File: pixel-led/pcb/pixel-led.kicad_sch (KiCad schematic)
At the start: 16 parts, among them J1 Conn_01x04_Socket, J2 USB_A, SW2 SW_Push, U1 AMS1117-3.3, U2 TSOP45xx, U3 ESP32-S3-MINI-1U, U4 USBLC6-2SC6

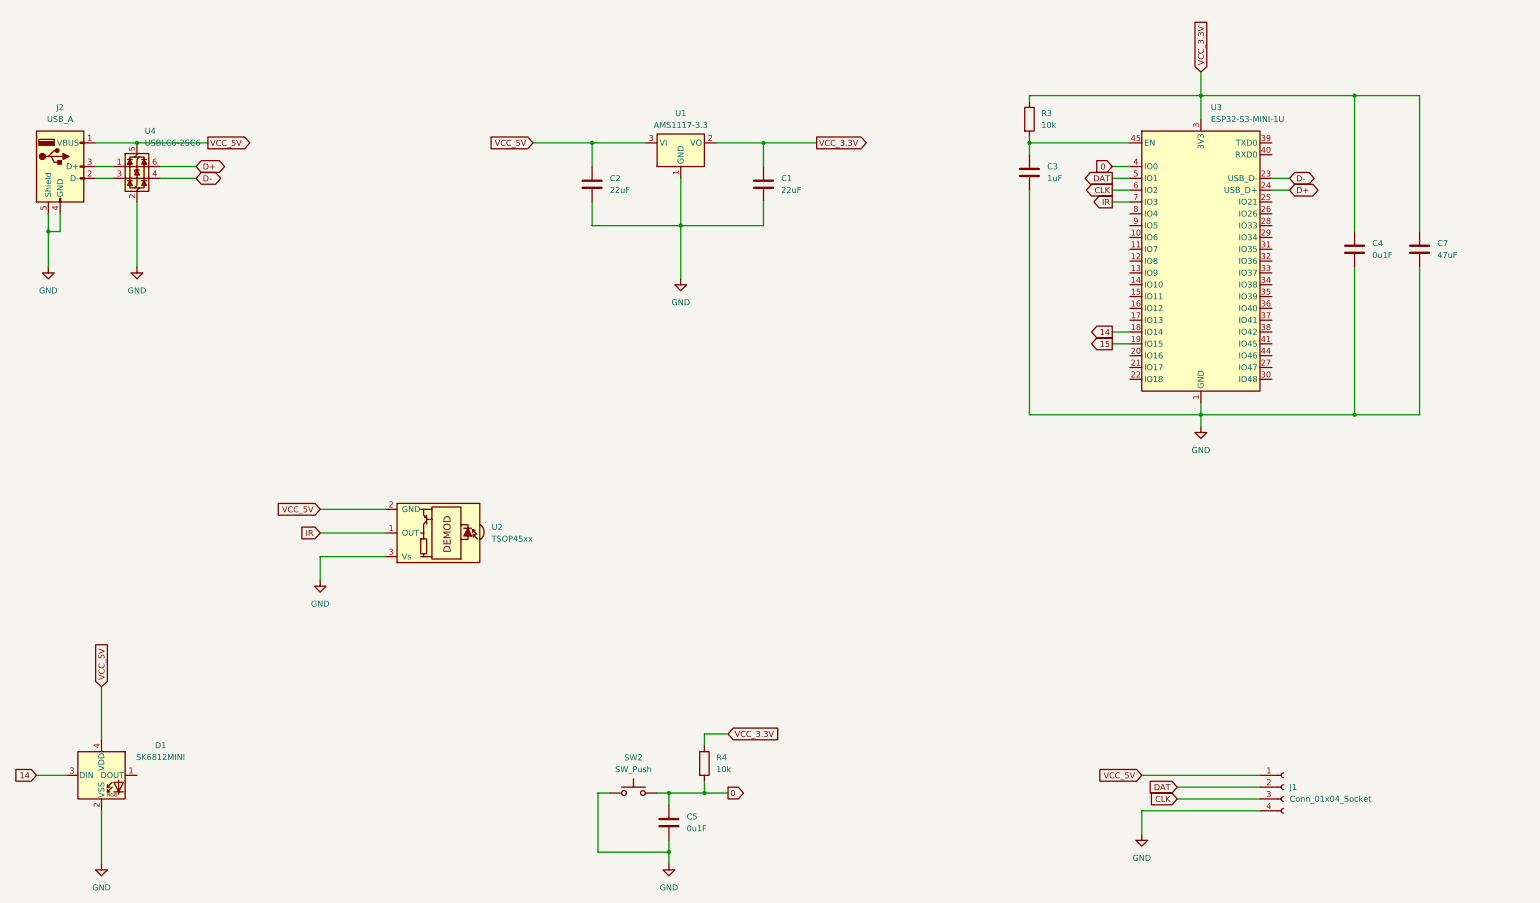
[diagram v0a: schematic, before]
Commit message: finishing layout
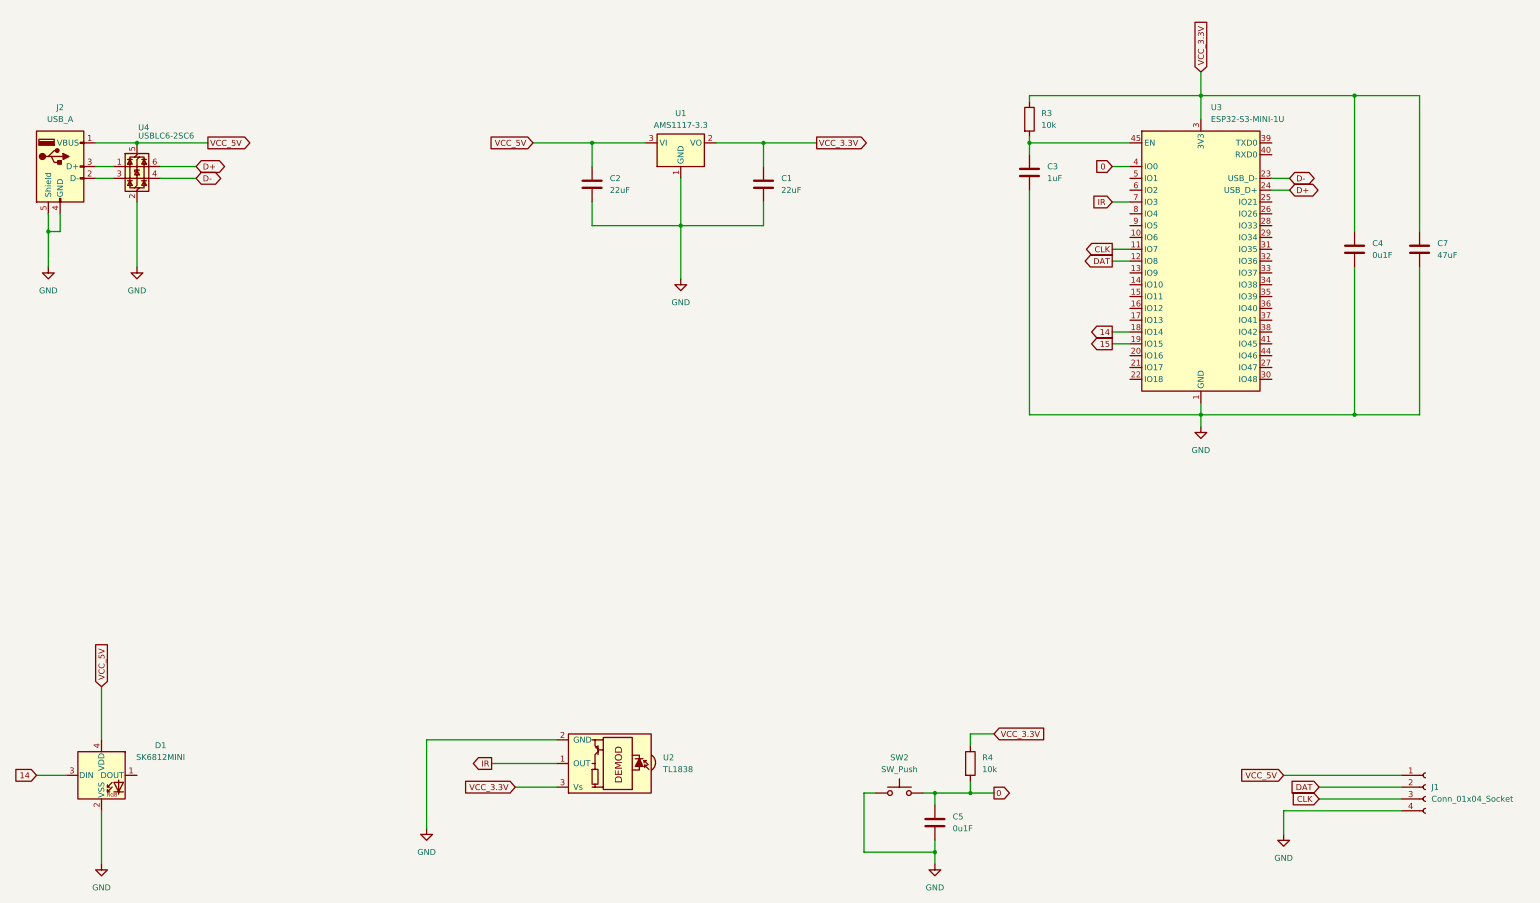
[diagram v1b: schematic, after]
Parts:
- U2: value TSOP45xx -> TL1838; ALIEXPRESS (none) -> https://de.aliexpress.com/item/1005004921187704.html
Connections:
- net CLK: now also U3.11 (IO7); no longer U3.6 (IO2)
- net DAT: now also U3.12 (IO8); no longer U3.5 (IO1)
- net GND: now also U2.2 (GND); no longer U2.3 (Vs)
- net VCC_3.3V: now also U2.3 (Vs)
- net VCC_5V: no longer U2.2 (GND)
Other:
- moved on the sheet: C5, J1, R4, SW2, U2
